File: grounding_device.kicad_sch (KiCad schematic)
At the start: 142 parts, among them IC1 NE555P, IC2 NE555P, IC3 NE555P, IC4 NE555P, Q1 2N2222, Q10 2N2222, Q11 2N2222, Q12 2N2222, Q2 2N2222, Q3 2N2222, Q4 2N2222, Q5 2N2222, Q6 2N2222, Q7 2N2222, Q8 2N2222, Q9 2N2222

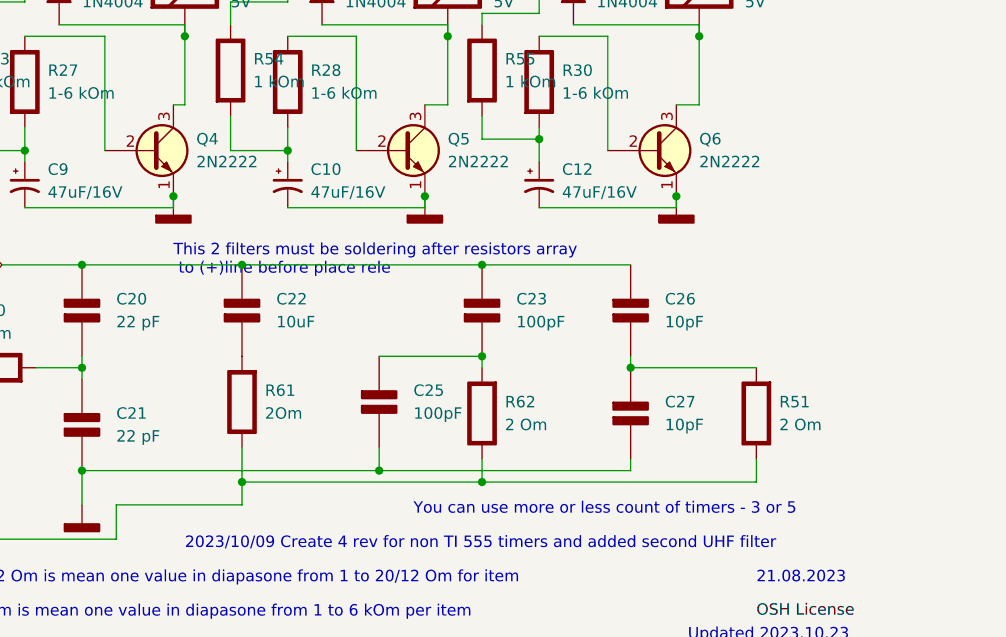
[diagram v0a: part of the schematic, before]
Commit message: Upgrade
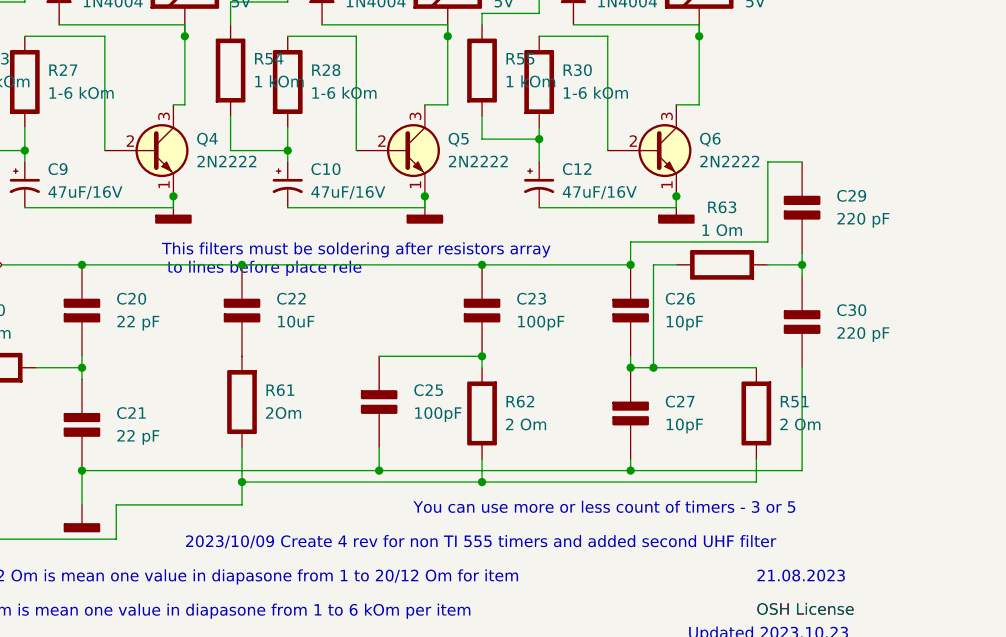
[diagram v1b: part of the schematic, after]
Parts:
- added C29, C30: 220 pF, symbol PCM_Elektuur:C
- added R63: 1 Om, symbol PCM_Elektuur:R
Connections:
- net 0: now also C30.2 (-)
- net To Reley 5v line : now also C29.1 (+)
- net at C26.2 (-), C27.1 (+), R51.2 (-): now also R63.1 (+)
- new net: C29.2 (-), C30.1 (+), R63.2 (-)
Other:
- note added: "This filters must be soldering after resistors array to lines before place rele"
- note removed: "This 2 filters must be soldering after resistors array to (+)line before place rele"
